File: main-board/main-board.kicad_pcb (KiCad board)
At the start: 2 copper layers, 100.7 x 67.1 mm, 62 parts, among them J1 16-bit, J2 7-12V, Q11 MBT3904DW1, Q12 MBT3904DW1, Q13 MBT3904DW1, Q14 MBT3904DW1, Q15 MBT3904DW1, Q16 MBT3904DW1, Q17 MBT3904DW1, Q18 MBT3904DW1, U1 CD40106BM96, U2 CD4024BM96, U3 CD4040BNSR, U4 27C256, U5 CD4028BM96, U6 KA78M05_TO252

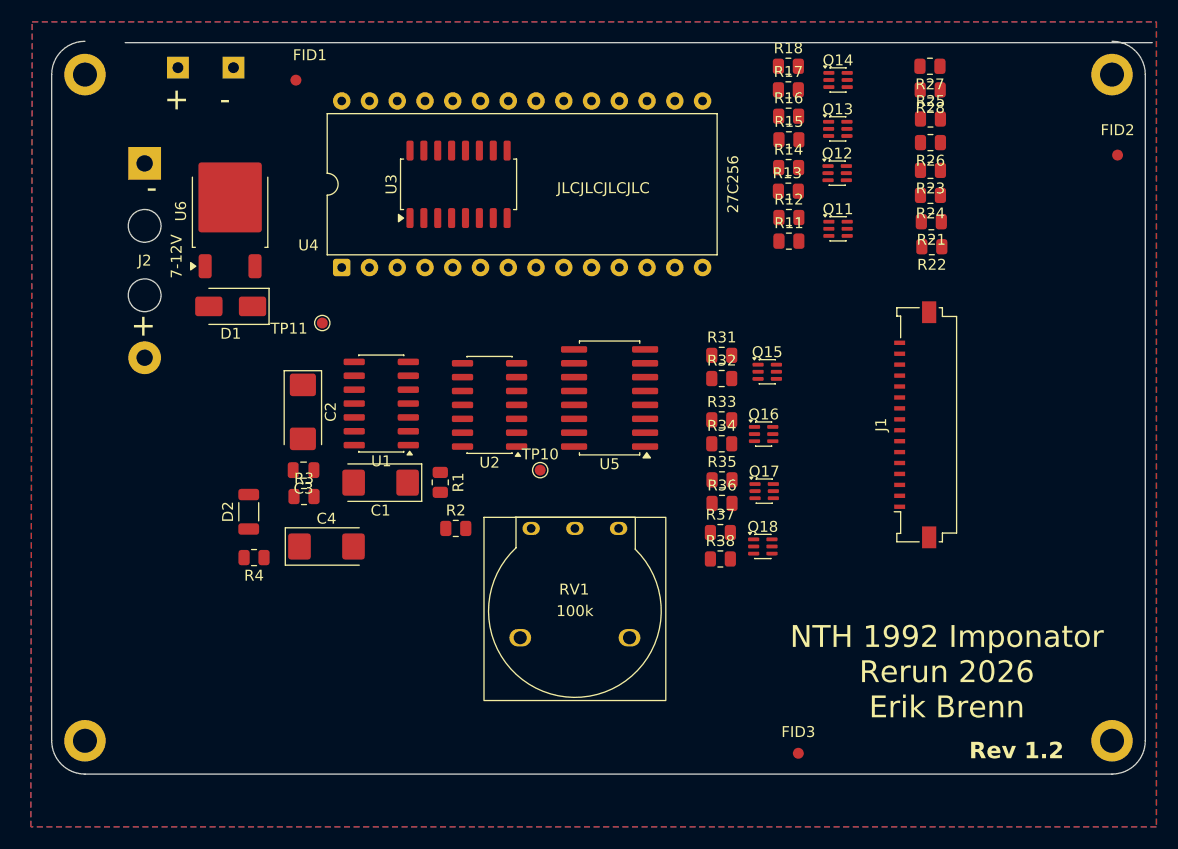
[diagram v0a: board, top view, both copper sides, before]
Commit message: routing complete - ready for QA
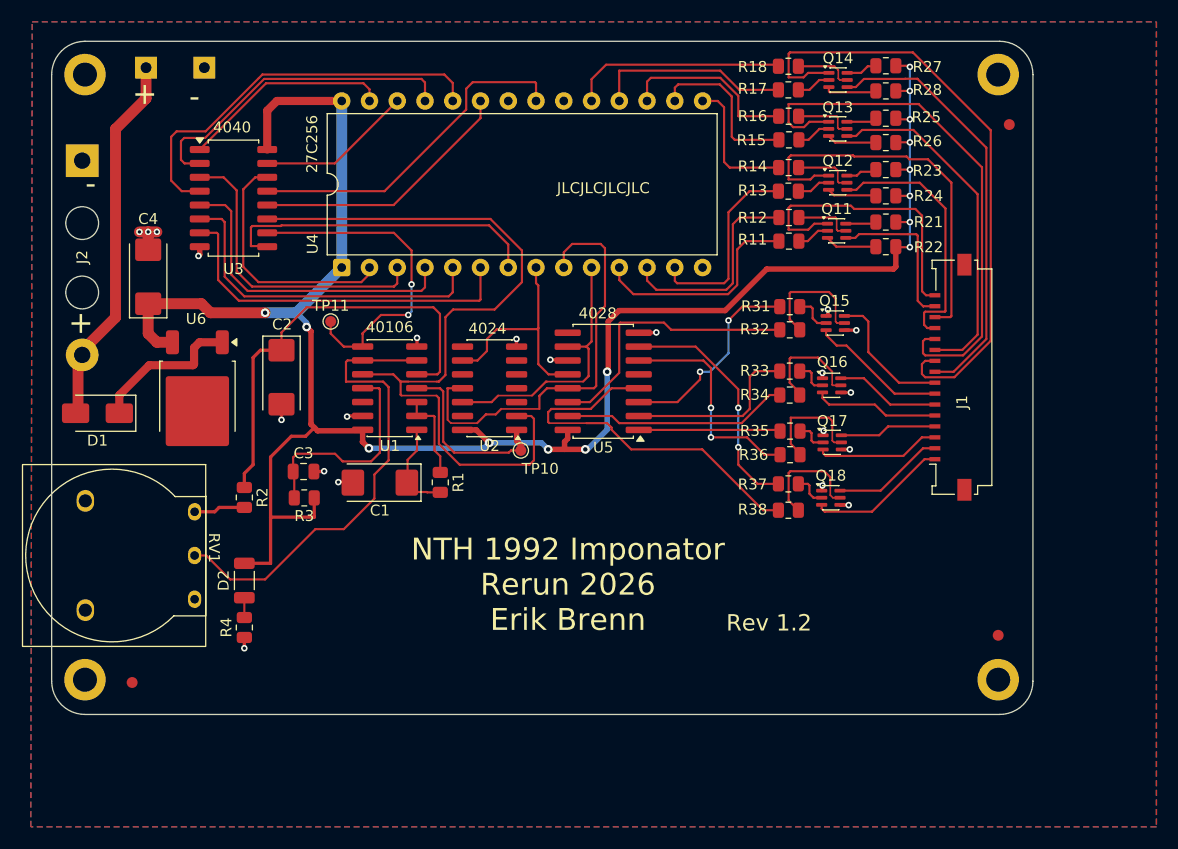
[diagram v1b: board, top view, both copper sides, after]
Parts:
- J2: footprint ezee-footprints:Battery_Terminals -> kicad-ezee-footprints:Battery_Terminals
- RV1: footprint ezee-footprints:Potentiometer_Wheel_3pin_Pitch4mm -> kicad-ezee-footprints:Potentiometer_Wheel_3pin_Pitch4mm
- TP10, TP11: footprint ezee-footprints:TestPoint_Pad_D1.0mm -> kicad-ezee-footprints:TestPoint_Pad_D1.0mm
- TPH1, TPH2: footprint ezee-footprints:TestPoint_Hook -> kicad-ezee-footprints:TestPoint_Hook
- moved FID1 65.4 mm to (187.2, 65.3)
- moved FID3 61.3 mm to (106.9, 116.3)
- moved FID2 45.3 mm to (186.2, 112.0)
- moved RV1 30.8 mm to (112.6, 100.7), turned to -90 degrees
- moved C4 29.6 mm to (108.4, 79.2), turned to 90 degrees
- moved U3 20.6 mm to (116.2, 72.0), turned to 0 degrees
- moved R2 19.6 mm to (117.2, 99.4), turned to -90 degrees
- moved U6 17.3 mm to (112.9, 90.2), turned to -90 degrees
- moved D1 15.6 mm to (103.8, 91.7)
- moved MH3 11.8 mm to (186.2, 116.1)
- moved MH4 10.4 mm to (186.2, 60.7)
- moved Q15 7.66 mm to (171.3, 83.4)
- moved Q16 7.66 mm to (170.9, 89.1)
- moved R35 7.66 mm to (167.1, 93.3)
- moved Q17 7.66 mm to (171.0, 94.4)
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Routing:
- net +5V: track 0.00 -> 186.7 mm, vias 0 -> 15
- net Net-(U2-MR): track 0.00 -> 73.3 mm
- net I7: track 0.00 -> 56.8 mm
- net I5: track 0.00 -> 49.8 mm
- net Net-(RV1-Pad2): track 0.00 -> 43.6 mm
- net Net-(C2-Pad1): track 0.00 -> 40.0 mm
- net I8: track 0.00 -> 39.1 mm
- net Net-(U2-Q1): track 0.00 -> 38.7 mm
- net Net-(U3-Q6): track 0.00 -> 37.1 mm
- net I3: track 0.00 -> 35.6 mm
- net Net-(U5-S7): track 0.00 -> 34.6 mm
- net Net-(D1-A): track 0.00 -> 34.3 mm
- net Net-(U3-Q1): track 0.00 -> 33.7 mm
- net I6: track 0.00 -> 32.0 mm
- net Net-(U3-Q7): track 0.00 -> 31.5 mm
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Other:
- board size 100.7 x 67.1 mm -> 89.8 x 61.6 mm
